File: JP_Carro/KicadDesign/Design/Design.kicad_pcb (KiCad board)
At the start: 2 copper layers, 130.4 x 40 mm, 14 parts, among them J10 Puente_H2, J11 A MOTOR, J12 B MOTOR, J13 SENSOR_SOURCE, J5 SENSOR, J6 Conn_01x20_Socket, J7 Conn_01x20_Socket, J8 Puente H, J9 9V, U3.3V1 LM317_TO-220

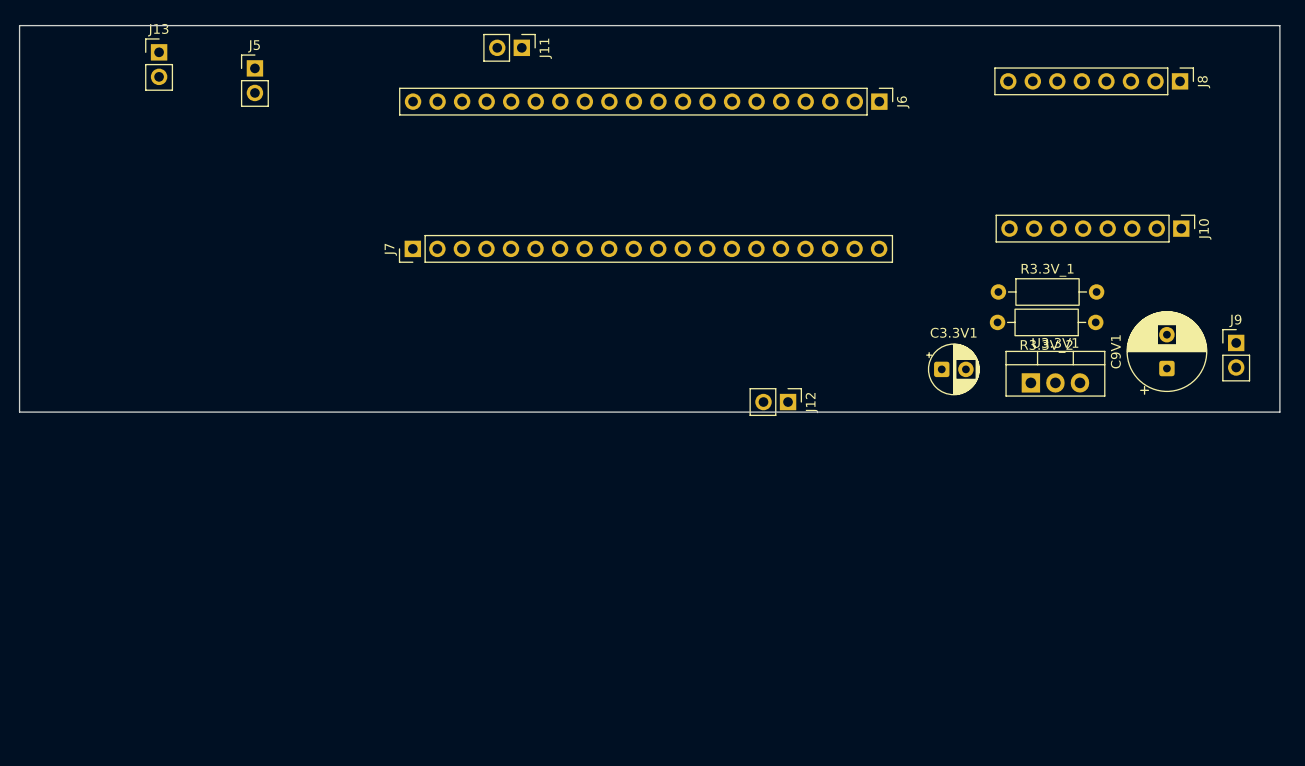
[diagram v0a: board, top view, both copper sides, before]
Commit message: PCB full
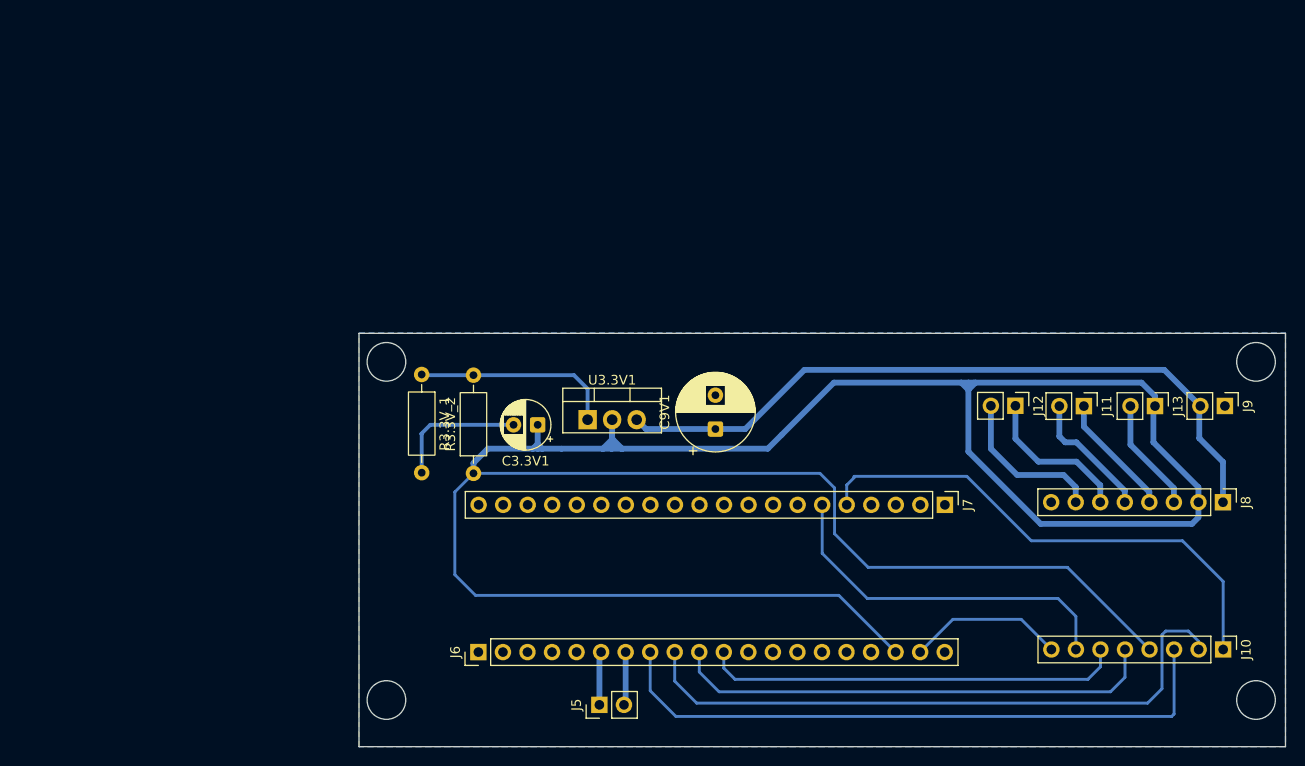
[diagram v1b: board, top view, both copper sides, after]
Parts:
- moved J13 109.4 mm to (156.4, 116.4), turned to -90 degrees
- moved J5 74.9 mm to (98.9, 147.3), turned to 90 degrees
- moved J6 70.5 mm to (86.4, 141.8), turned to 90 degrees
- moved J11 69.0 mm to (149.0, 116.4)
- moved R3.3V_2 66.3 mm to (85.9, 123.3), turned to 90 degrees
- moved J7 61.1 mm to (134.7, 126.6), turned to -90 degrees
- moved R3.3V_1 60.3 mm to (80.5, 113.1), turned to -90 degrees
- moved C9V1 47.1 mm to (110.9, 118.8)
- moved U3.3V1 46.0 mm to (97.7, 117.8)
- moved J8 43.8 mm to (163.4, 126.3)
- moved J10 43.8 mm to (163.5, 141.6)
- moved C3.3V1 42.2 mm to (92.5, 118.3), turned to 180 degrees
- moved J12 23.5 mm to (142.0, 116.3)
- moved J9 6.63 mm to (163.6, 116.4), turned to -90 degrees
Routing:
- net 3.3V: track 0.00 -> 277.4 mm
- net 9V: track 0.00 -> 73.8 mm
- net A2 AIN1: track 0.00 -> 66.1 mm
- net A3 AIN2: track 0.00 -> 65.8 mm
- net A8 PWM_IZQ: track 0.00 -> 53.0 mm
- net A4 BIN1: track 0.00 -> 50.5 mm
- net A5 BIN2: track 0.00 -> 43.4 mm
- net GND: track 0.00 -> 42.1 mm
- net A9 PWM_DER: track 0.00 -> 37.4 mm
- net Net-(U3.3V1-ADJ): track 0.00 -> 21.0 mm
- net /B02: track 0.00 -> 17.0 mm
- net /B01: track 0.00 -> 15.9 mm
- net /A02: track 0.00 -> 13.4 mm
- net /A01: track 0.00 -> 12.8 mm
- net A1 ADC_2: track 0.00 -> 5.53 mm
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- added copper zone on B.Cu, net GND
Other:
- board size 130.4 x 40 mm -> 95.9 x 42.8 mm

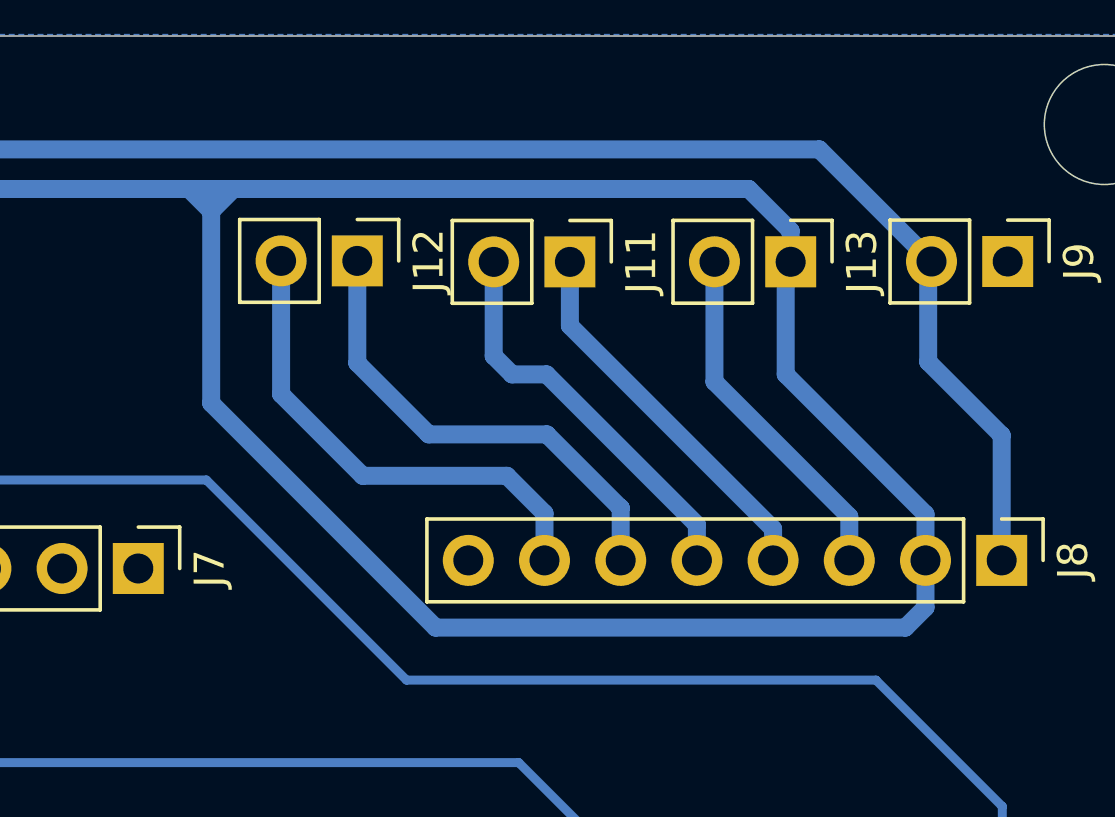
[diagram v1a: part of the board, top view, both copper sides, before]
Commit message: Readme 1
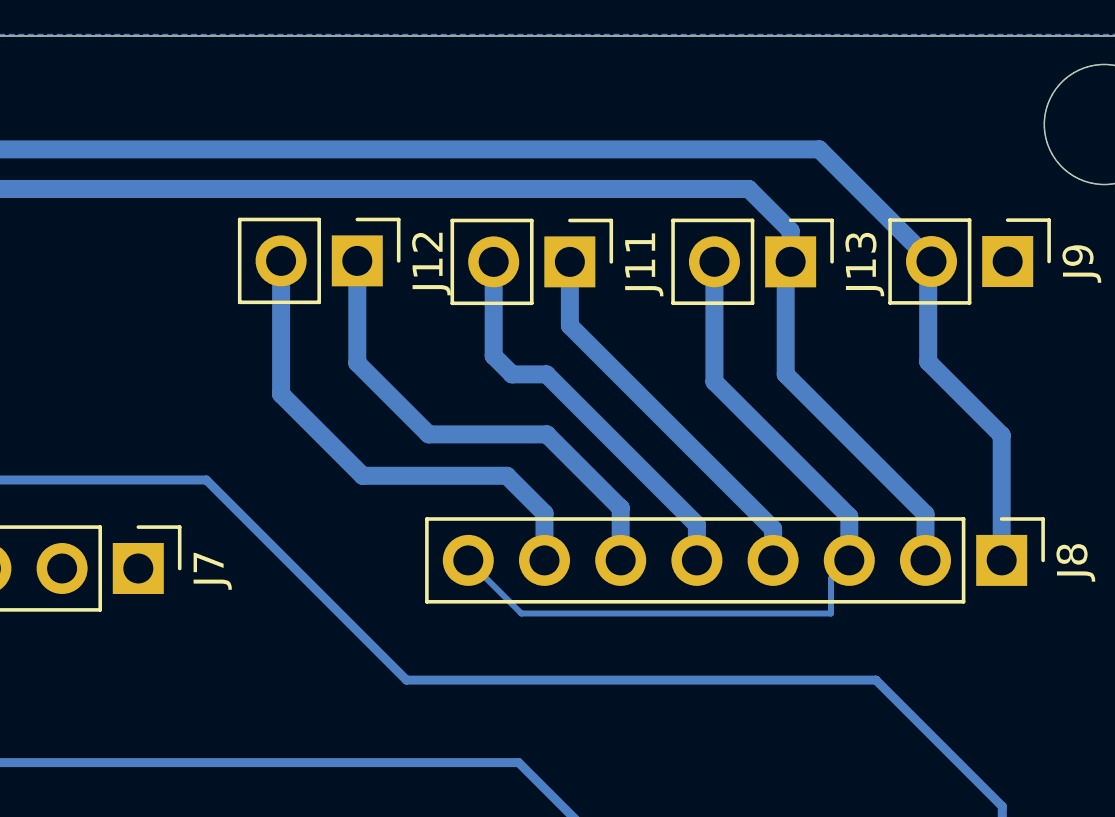
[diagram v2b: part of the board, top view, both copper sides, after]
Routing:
- net 3.3V: track 277.4 -> 239.2 mm
- net GND: track 42.1 -> 56.9 mm
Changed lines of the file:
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@@
+	)
+	(segment
+		(start 157.75 126.94)
+		(end 158.36 126.33)
+		(width 0.2)
+		(layer "B.Cu")
+		(net "GND")
 	)
 	(segment
@@
 	)
 	(segment
+		(start 157.75 128.1)
+		(end 157.75 126.94)
+		(width 0.2)
+		(layer "B.Cu")
+		(net "GND")
+	)
+	(segment
 		(start 81.402651 118.317349)
 		(end 80.48 119.24)
@@
 	)
 	(segment
+		(start 147.43 128.1)
+		(end 157.75 128.1)
+		(width 0.2)
+		(layer "B.Cu")
+		(net "GND")
+	)
+	(segment
 		(start 142.56 138.45)
 		(end 145.68 141.57)
@@
 		(end 158.36 124.87)
 		(width 0.6)
+		(layer "B.Cu")
+		(net "GND")
+	)
+	(segment
+		(start 145.66 126.33)
+		(end 147.43 128.1)
+		(width 0.2)
 		(layer "B.Cu")
 		(net "GND")
@@
 	)
 	(segment
-		(start 144.57 128.57)
-		(end 137.09 121.09)
-		(width 0.6)
-		(layer "B.Cu")
-		(net "3.3V")
-	)
-	(segment
-		(start 137.09 114.69)
-		(end 137.83 113.95)
-		(width 0.6)
-		(layer "B.Cu")
-		(net "3.3V")
-	)
-	(segment
 		(start 100.22 120.75)
 		(end 100.22 119.417349)
@@
 	)
 	(segment
-		(start 137.09 114.69)
-		(end 137.09 113.95)
-		(width 0.6)
-		(layer "B.Cu")
-		(net "3.3V")
-	)
-	(segment
-		(start 137.09 121.09)
-		(end 137.09 114.69)
-		(width 0.6)
-		(layer "B.Cu")
-		(net "3.3V")
-	)
-	(segment
-		(start 160.23 128.57)
-		(end 144.57 128.57)
-		(width 0.6)
-		(layer "B.Cu")
-		(net "3.3V")
-	)
-	(segment
 		(start 160.9 124.79)
 		(end 160.9 126.33)
@@
 	)
 	(segment
-		(start 137.09 114.69)
-		(end 137.09 114.5)
-		(width 0.6)
-		(layer "B.Cu")
-		(net "3.3V")
-	)
-	(segment
 		(start 100.182651 120.787349)
 		(end 101.25 120.787349)
@@
 	)
 	(segment
-		(start 160.9 127.9)
-		(end 160.23 128.57)
-		(width 0.6)
-		(layer "B.Cu")
-		(net "3.3V")
-	)
-	(segment
 		(start 137.64 113.95)
 		(end 137.09 113.95)
@@
 		(width 0.6)
 		(layer "B.Cu")
-		(net "3.3V")
-	)
-	(segment
-		(start 137.09 114.69)
-		(end 136.35 113.95)
-		(width 0.6)
-		(layer "B.Cu")
-		(net "3.3V")
-	)
-	(segment
-		(start 160.9 126.33)
-		(end 160.9 127.9)
-		(width 0.6)
-		(layer "B.Cu")
